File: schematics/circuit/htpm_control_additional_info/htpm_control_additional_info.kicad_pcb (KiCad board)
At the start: 2 copper layers, 99.1 x 82 mm, 66 parts, among them J1 Conn_01x10_Socket, J2 Conn_01x04_Socket, J3 Conn_01x04_Socket, J4 Conn_01x08_Socket, J5 Conn_01x08_Socket, J6 Conn_01x04_Socket, J7 Conn_01x04_Socket, J8 Conn_01x08_Socket, J9 Conn_01x05_Socket, U1 L7805, U2 74HC595, U3 74HC595, U4 74HC595, U5 74HC595, U6 MAX7219, U7 MAX7219

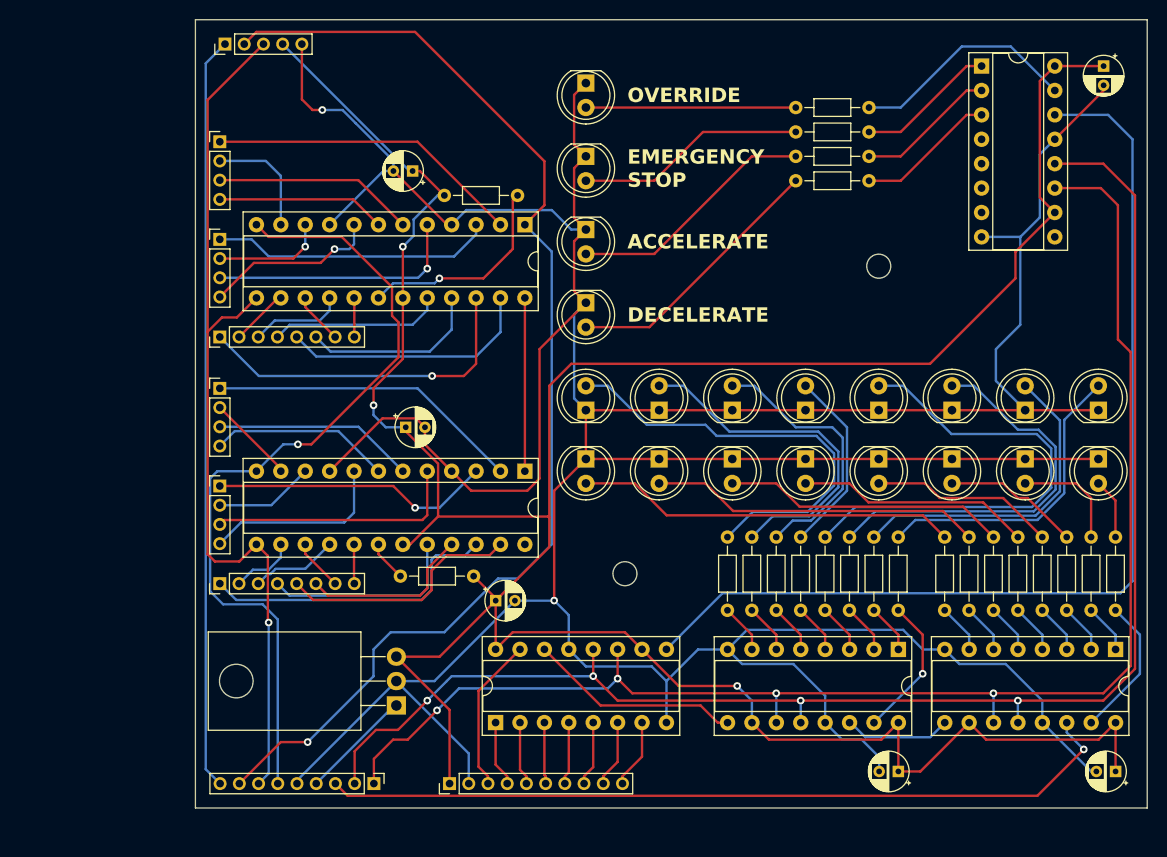
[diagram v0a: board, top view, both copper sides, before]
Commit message: Updated annotations.
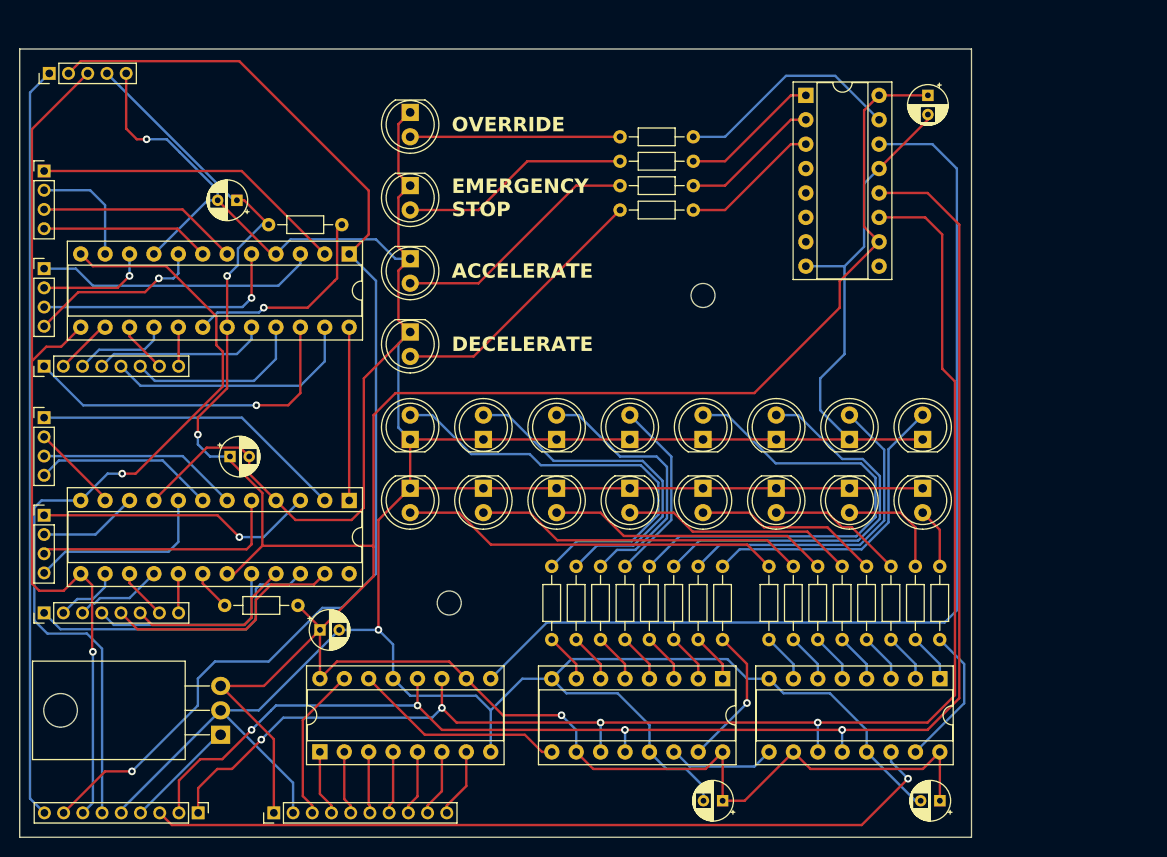
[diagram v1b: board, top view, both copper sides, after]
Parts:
- moved J1 18.5 mm to (119.9, 128.3)
- moved C2 18.5 mm to (166.6, 127.0)
- moved C4 18.5 mm to (188.0, 53.6)
- moved C5 18.5 mm to (116.1, 64.5)
- moved D1 18.5 mm to (134.1, 55.4)
- moved D11 18.5 mm to (141.7, 89.4)
- moved D12 18.5 mm to (134.1, 89.4)
- moved D13 18.5 mm to (187.5, 94.5)
- moved D14 18.5 mm to (179.8, 94.5)
- moved D15 18.5 mm to (172.2, 94.5)
- moved D19 18.5 mm to (141.7, 94.5)
- moved D2 18.5 mm to (134.1, 63.0)
- moved D20 18.5 mm to (134.1, 94.5)
- moved D3 18.5 mm to (134.1, 70.6)
- moved D4 18.5 mm to (134.1, 78.2)
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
